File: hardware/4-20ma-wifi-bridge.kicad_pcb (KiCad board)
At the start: 2 copper layers, 32 x 83 mm, 16 parts, among them J1 Conn_01x19_Female, J2 Conn_01x19_Female, J3 Screw_Terminal_01x02, J4 Screw_Terminal_01x02, M1 DC-DC_Buck_Step_Module-dc-dc_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, SW1 SW_DIP_x01, U1 ESP32-DEVKITC-32D, U2 INA196

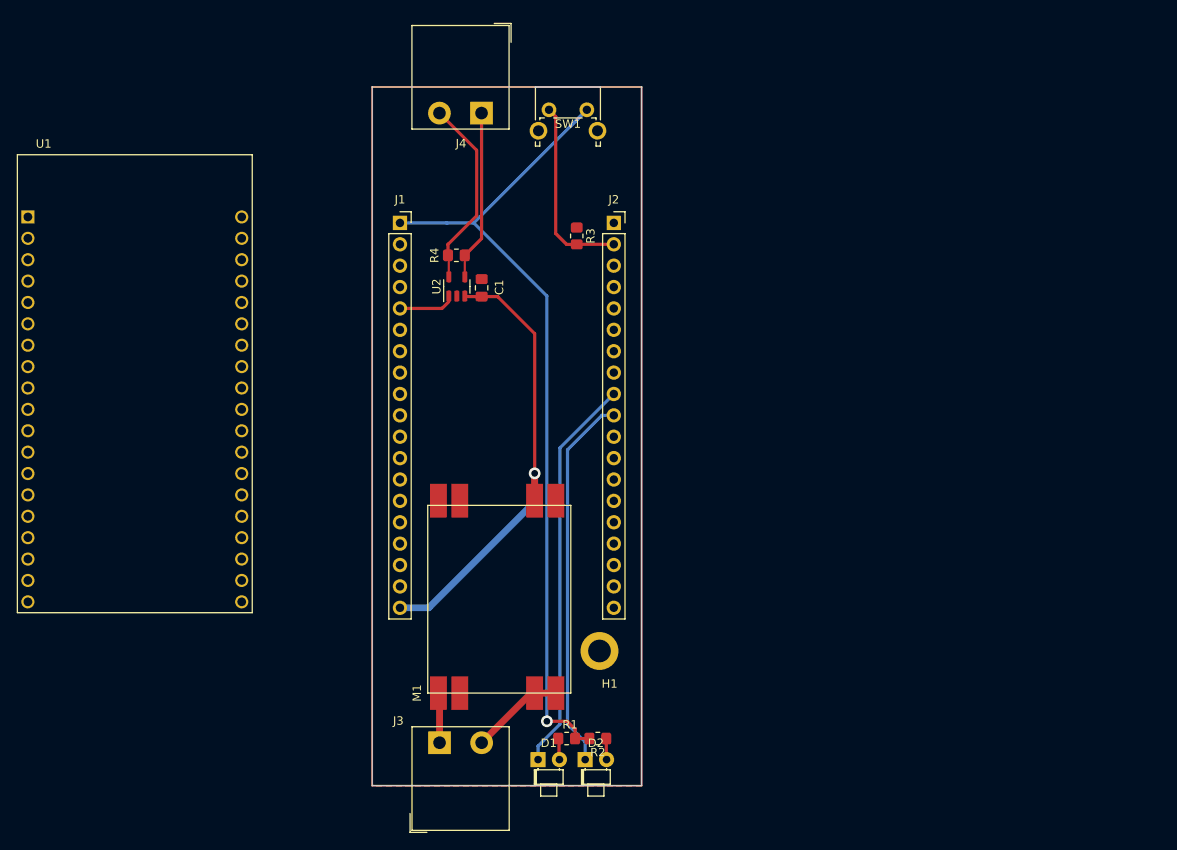
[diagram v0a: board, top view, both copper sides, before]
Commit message: Added kicad design files
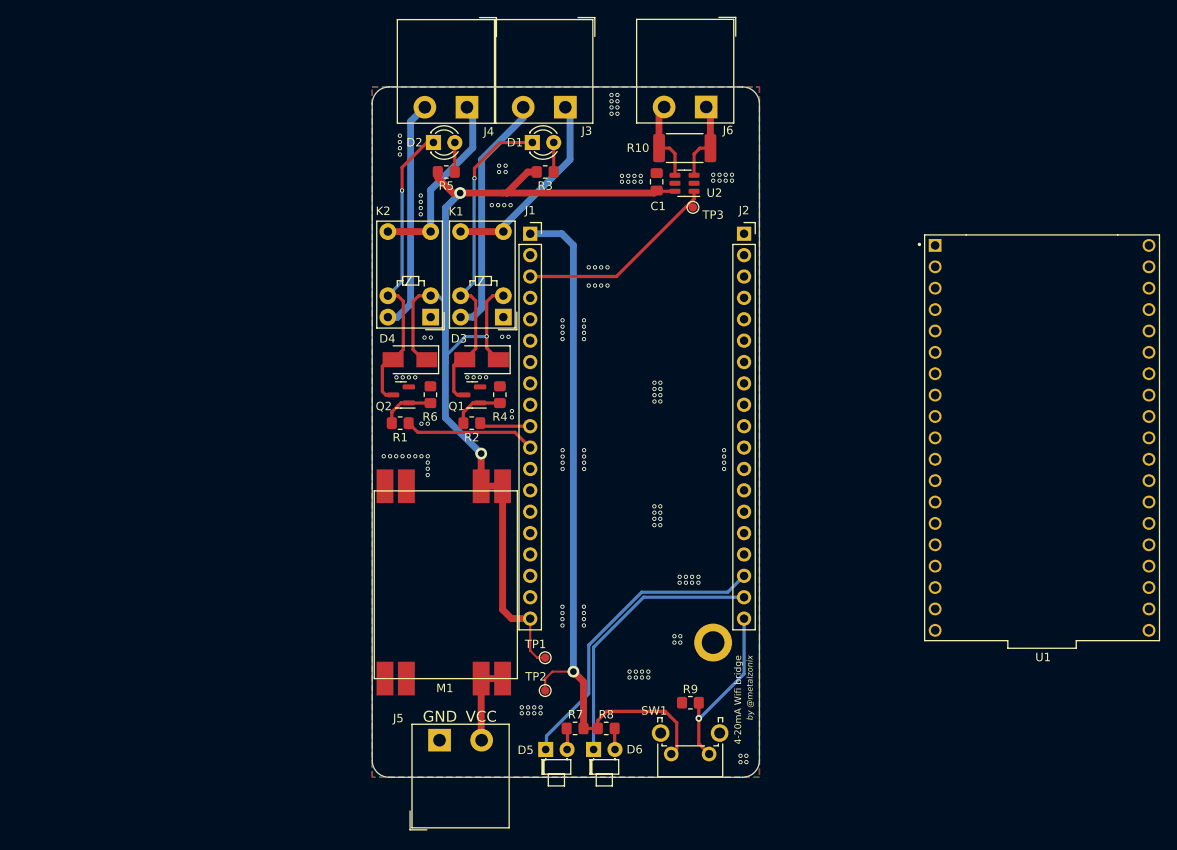
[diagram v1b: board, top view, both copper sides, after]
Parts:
- added D2: LED, LED_THT:LED_D3.0mm_FlatTop, F.Cu at (145.3, 47.6)
- added D3: 1N4004, Diode_SMD:D_SMA, F.Cu at (151.0, 73.4)
- added D4: 1N4004, Diode_SMD:D_SMA, F.Cu at (142.5, 73.4)
- added D5: LED, LED_THT:LED_D1.8mm_W1.8mm_H2.4mm_Horizontal_O1.27mm_Z1.6mm, F.Cu at (158.6, 119.7)
- added J3: Screw_Terminal_01x02, project_library:TerminalBlock__1x02_P5.00mm_90Degree, F.Cu at (160.9, 43.4)
- added J4: Screw_Terminal_01x02, project_library:TerminalBlock__1x02_P5.00mm_90Degree, F.Cu at (149.3, 43.4)
- added K1: G5V-1, Relay_THT:Relay_SPDT_Omron_G5V-1, F.Cu at (153.6, 68.3)
- added K2: G5V-1, Relay_THT:Relay_SPDT_Omron_G5V-1, F.Cu at (144.9, 68.3)
- added Q1: 2N7002E, Package_TO_SOT_SMD:SOT-23, F.Cu at (149.9, 77.6)
- added Q2: 2N7002E, Package_TO_SOT_SMD:SOT-23, F.Cu at (141.4, 77.6)
- added R1: 1k, Resistor_SMD:R_0805_2012Metric_Pad1.20x1.40mm_HandSolder, F.Cu at (141.3, 80.9)
- added R2: 1k, Resistor_SMD:R_0805_2012Metric_Pad1.20x1.40mm_HandSolder, F.Cu at (149.8, 80.9)
- added R3: 1k, Resistor_SMD:R_0805_2012Metric_Pad1.20x1.40mm_HandSolder, F.Cu at (158.6, 51.1)
- added R4: 10k, Resistor_SMD:R_0805_2012Metric_Pad1.20x1.40mm_HandSolder, F.Cu at (153.2, 77.6)
- added R5: 1k, Resistor_SMD:R_0805_2012Metric_Pad1.20x1.40mm_HandSolder, F.Cu at (146.8, 51.1)
- added R6: 10k, Resistor_SMD:R_0805_2012Metric_Pad1.20x1.40mm_HandSolder, F.Cu at (144.9, 77.6)
- added TP1: TestPoint, TestPoint:TestPoint_Pad_D1.0mm, F.Cu at (158.6, 108.8)
- added TP2: TestPoint, TestPoint:TestPoint_Pad_D1.0mm, F.Cu at (158.6, 112.7)
- added TP3: TestPoint, TestPoint:TestPoint_Pad_D1.0mm, F.Cu at (176.1, 55.3)
- D1: footprint LED_THT:LED_D1.8mm_W1.8mm_H2.4mm_Horizontal_O1.27mm_Z4.9mm -> LED_THT:LED_D3.0mm_FlatTop
- R10: renamed from R4; value 4.99 -> 2.7ohm; footprint Resistor_SMD:R_0805_2012Metric_Pad1.20x1.40mm_HandSolder -> Resistor_SMD:R_2512_6332Metric_Pad1.40x3.35mm_HandSolder
- R7: renamed from R1; value 250 -> 1k
- R8: renamed from R2; value 250 -> 1k
- R9: renamed from R3; value 4.99 -> 10k
- U1: value ESP32-DEVKITC-32D -> ESP32-DEVKITC-32U; footprint project_library:MODULE_ESP32-DEVKITC-32D -> project_library:MODULE_ESP32-DEVKITC-32U
- U2: value INA196 -> LMP8640; footprint Package_TO_SOT_SMD:SOT-23-5 -> Package_TO_SOT_SMD:SOT-23-6
- moved U1 108.0 mm to (217.6, 82.7)
- moved SW1 78.9 mm to (178.0, 120.2), turned to 180 degrees
- moved D1 73.3 mm to (157.0, 47.6)
- moved R9 57.1 mm to (175.8, 114.2), turned to 0 degrees
- moved R10 30.0 mm to (175.1, 48.3)
- moved U2 29.7 mm to (175.1, 52.4), turned to 180 degrees
- moved J6 26.7 mm to (177.7, 43.4)
- moved C1 24.3 mm to (171.8, 52.3)
- moved J1 15.5 mm to (156.8, 58.4)
- moved J2 15.5 mm to (182.2, 58.4)
- moved H1 13.5 mm to (178.5, 107.0)
- moved M1 6.58 mm to (138.2, 111.3)
- moved D6 1.56 mm to (164.3, 119.7)
- moved R7 1.56 mm to (162.1, 117.2)
- moved R8 1.56 mm to (165.8, 117.2)
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- renumbered D2 to D6, J3 to J5, J4 to J6
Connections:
- D1 pad 1: led1 -> Net-(D1-Pad1)
- J1 pad 10: unconnected-(J1-Pad10) -> relay1
- J1 pad 11: unconnected-(J1-Pad11) -> relay2
- J1 pad 3: unconnected-(J1-Pad3) -> vsens
- J1 pad 5: vsens -> unconnected-(J1-Pad5)
- J2 pad 10: led2 -> unconnected-(J2-Pad10)
- J2 pad 17: unconnected-(J2-Pad17) -> led1
- J2 pad 18: unconnected-(J2-Pad18) -> led2
- J2 pad 19: unconnected-(J2-Pad19) -> switch
- J2 pad 2: switch -> unconnected-(J2-Pad2)
- J2 pad 9: led1 -> unconnected-(J2-Pad9)
- J6 pad 1: Net-(R4-Pad1) -> Net-(J6-Pad1)
- J6 pad 2: Net-(J4-Pad2) -> Net-(J6-Pad2)
- R10 pad 1: Net-(R4-Pad1) -> Net-(J6-Pad1)
- R10 pad 2: Net-(J4-Pad2) -> Net-(J6-Pad2)
- R7 pad 1: Net-(D1-Pad2) -> Net-(D5-Pad2)
- U2 pad 3: +5V -> Net-(J6-Pad1)
- U2 pad 4: Net-(R4-Pad1) -> Net-(J6-Pad2)
- U2 pad 5: Net-(J4-Pad2) -> (no net)
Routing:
- net +5V: track 54.6 -> 126.5 mm, vias 1 -> 3
- net Net-(D1-Pad1): track 0.00 -> 39.7 mm, vias 0 -> 1
- net Net-(D2-Pad1): track 0.00 -> 38.4 mm, vias 0 -> 1
- net Net-(J3-Pad2): track 0.00 -> 28.9 mm
- net Net-(J3-Pad1): track 0.00 -> 24.5 mm
- net Net-(J4-Pad1): track 0.00 -> 22.2 mm
- net Net-(R4-Pad1): track 20.3 -> 0.00 mm
- net vsens: track 6.80 -> 24.8 mm
- net relay2: track 0.00 -> 15.6 mm
- net +3V3: track 100.1 -> 85.8 mm
- net led2: track 44.9 -> 32.5 mm
- net led1: track 47.2 -> 36.3 mm
- net Net-(J6-Pad2): track 0.00 -> 10.0 mm
- net Net-(J6-Pad1): track 0.00 -> 9.86 mm
- net Net-(Q2-Pad1): track 0.00 -> 6.35 mm
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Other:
- board size 32 x 83 mm -> 46 x 82 mm
- board text added: "4-20mA Wifi bridge"
- board text added: "GND"
- board text added: "VCC"
- board text added: "by @metalzonix"
